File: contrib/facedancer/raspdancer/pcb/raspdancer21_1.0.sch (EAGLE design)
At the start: 15 parts, among them Q1 12Mhz, U1 MAX3421E

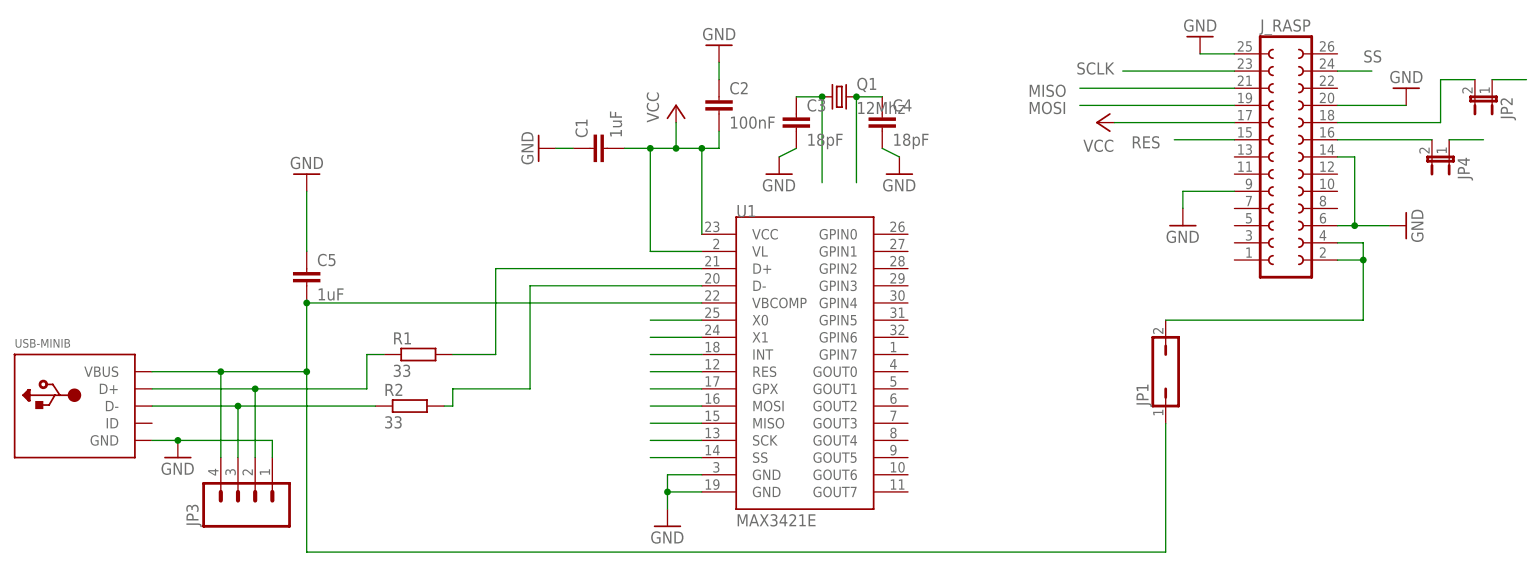
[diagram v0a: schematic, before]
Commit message: raspdancer pcb edited
thanks to Zac Franken for his tuning tips

git-svn-id: https://svn.code.sf.net/p/goodfet/code@1589 12e2690d-a6be-4b82-a7b7-67c4a43b65c8
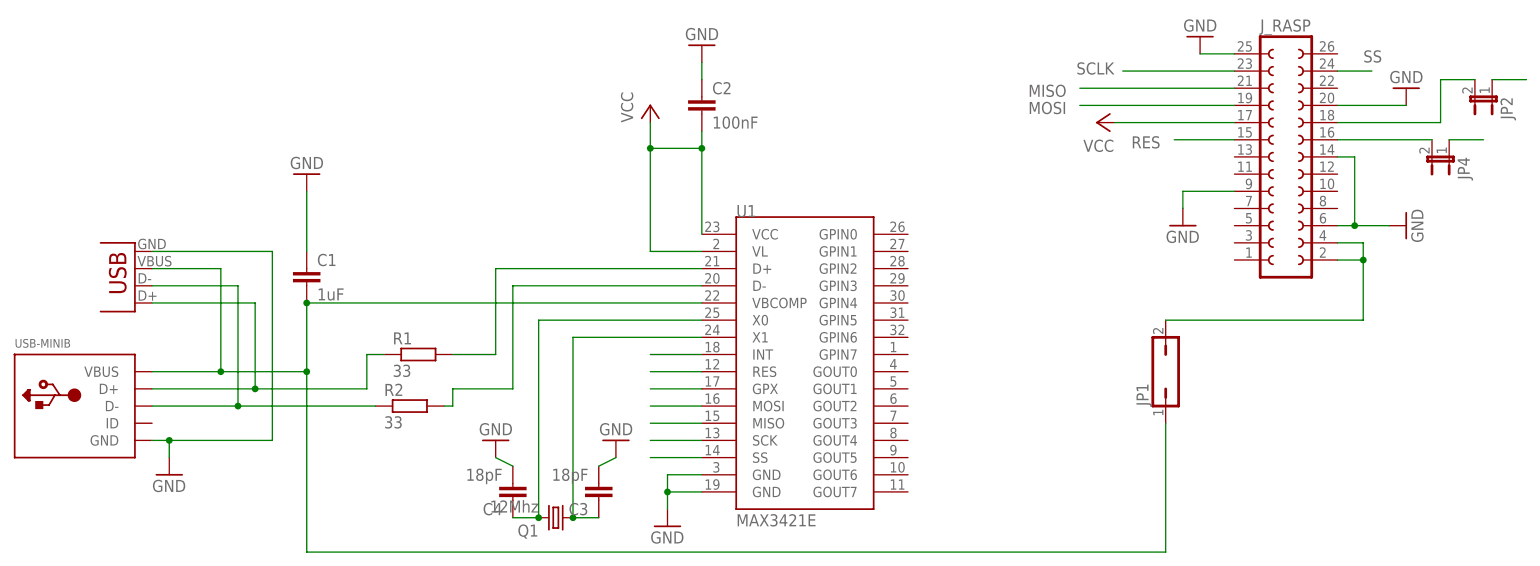
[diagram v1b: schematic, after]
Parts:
- removed C5: 1uF, 00_mylib:C1206
- removed JP3: (no value), SparkFun:M04PTH
- added JP5: USB-A-S, SparkFun-Connectors:USB-A-S
- J_RASP: device con-lsta:FE13-2 -> doegox:FE13-2
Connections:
- removed net VBCOMP: C5.2, JP1.1, JP3.4, U1.VBCOMP, USB-MINIB.VBUS
- new net VBUS: C1.2, JP1.1, JP5.VBUS, U1.VBCOMP, USB-MINIB.VBUS
- net D+2: now also JP5.D+; no longer JP3.2
- net D-2: now also JP5.D-; no longer JP3.3
- net GND: now also JP5.GND, USB-MINIB.GND; no longer C5.1, JP3.1
- net VCC: no longer C1.2
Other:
- moved on the sheet: C1, C2, C3, C4, Q1
